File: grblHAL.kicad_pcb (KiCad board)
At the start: 2 copper layers, 48 parts, among them J1 Conn_01x03, J2 Conn_02x08_Odd_Even, J3 Conn_01x06, J4 Conn_01x06, J5 Conn_01x04, U1 YAAJ_BluePill_Part_Like_SWD_B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, U10 PC817, U11 PC817, U12 PC817, U13 PC817, U14 LM1117-3.3, U2 TMC2208_SILENTSTEPSTICK, U4 PC817, U5 PC817, U6 PC817, U7 PC817, U8 PC817, U9 PC817

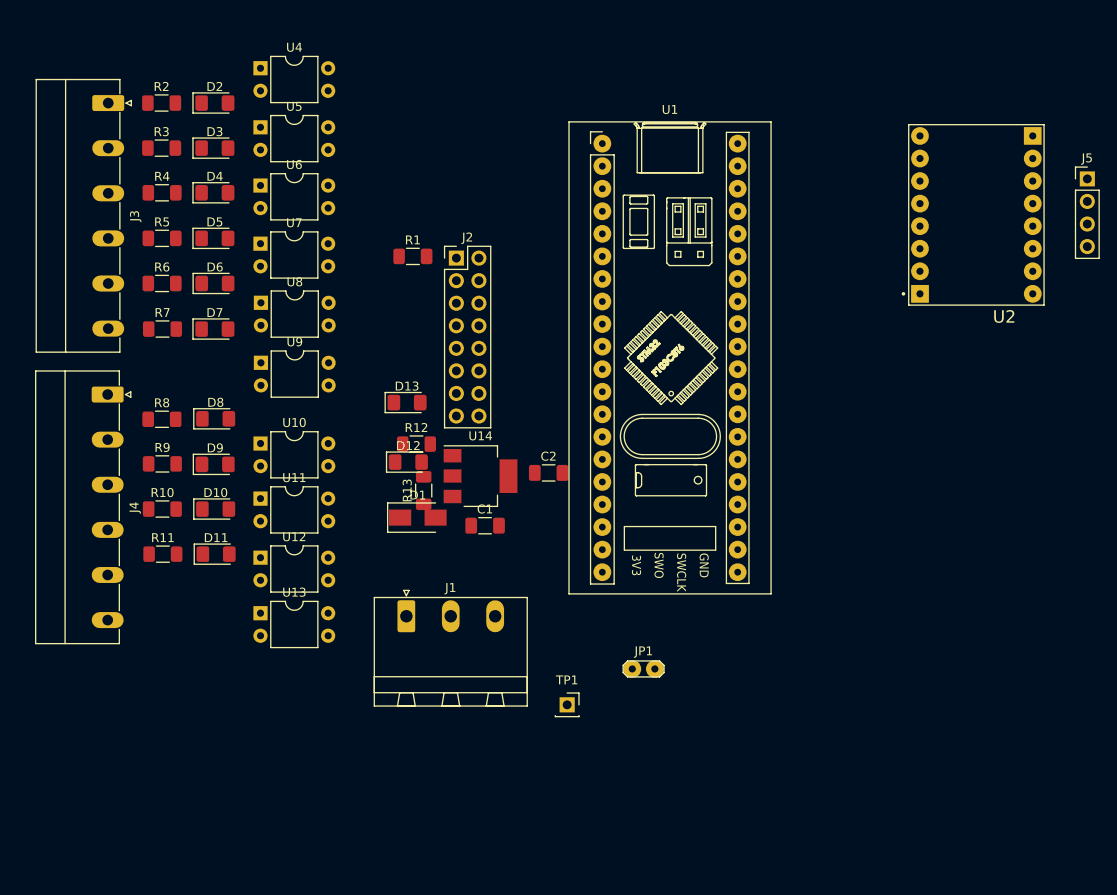
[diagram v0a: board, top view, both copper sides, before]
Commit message: Schematic Layout Nets Opto 4 TMC Stage 2
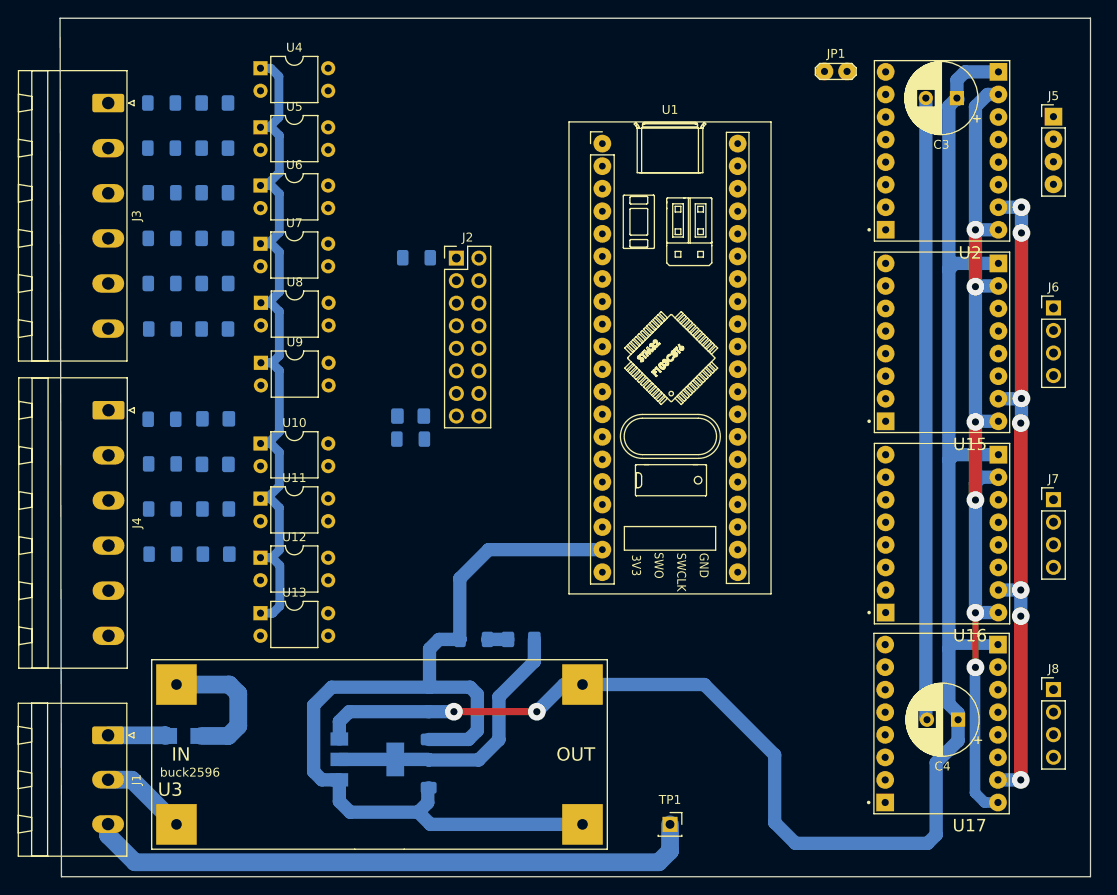
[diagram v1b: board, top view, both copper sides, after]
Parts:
- added C3: 100uF/35v, Capacitor_THT:CP_Radial_D8.0mm_P3.50mm, F.Cu at (156.1, 60.1)
- added C4: 100uF/35v, Capacitor_THT:CP_Radial_D8.0mm_P3.50mm, F.Cu at (156.2, 130.1)
- added J6: Conn_01x04, Connector_PinHeader_2.54mm:PinHeader_1x04_P2.54mm_Vertical, F.Cu at (166.9, 83.7)
- added J7: Conn_01x04, Connector_PinHeader_2.54mm:PinHeader_1x04_P2.54mm_Vertical, F.Cu at (166.9, 105.3)
- added J8: Conn_01x04, Connector_PinHeader_2.54mm:PinHeader_1x04_P2.54mm_Vertical, F.Cu at (166.9, 126.7)
- added U15: TMC2208, TMC2208_SILENTSTEPSTICK:MODULE_TMC2208_SILENTSTEPSTICK, F.Cu at (154.4, 87.6)
- added U16: TMC2208, TMC2208_SILENTSTEPSTICK:MODULE_TMC2208_SILENTSTEPSTICK, F.Cu at (154.4, 109.1)
- added U17: TMC2208, TMC2208_SILENTSTEPSTICK:MODULE_TMC2208_SILENTSTEPSTICK, F.Cu at (154.3, 130.5)
- added U3: buck2596, DC_DC_LM2596_small:DC_DC_LM2596_small, F.Cu at (91.0, 134.0)
- C1, C2, D1, D10, D11, D12, D13, D2, D3, D4, D5, D6, D7, D8, D9, R1, R10, R11, R12, R13, R2, R3, R4, R5, R6, R7, R8, R9, U14: moved to B.Cu
- J2: value Conn_02x08_Odd_Even -> Conn
- J3, J4: footprint Connector_Phoenix_MC_HighVoltage:PhoenixContact_MC_1,5_6-G-5.08_1x06_P5.08mm_Horizontal -> Connector_Phoenix_MSTB:PhoenixContact_MSTBA_2,5_6-G-5,08_1x06_P5.08mm_Horizontal
- U2: value TMC2208_SILENTSTEPSTICK -> TMC2208
- moved JP1 70.7 mm to (141.1, 57.1)
- moved C2 36.5 mm to (96.6, 136.2), turned to -90 degrees
- moved J1 36.2 mm to (60.5, 131.9), turned to -90 degrees
- moved D1 36.1 mm to (69.0, 131.9), turned to 180 degrees
- moved U14 34.4 mm to (89.7, 134.6)
- moved D12 23.7 mm to (107.0, 121.1)
- moved C1 23.4 mm to (96.6, 130.8), turned to -90 degrees
- moved TP1 17.8 mm to (123.7, 141.9)
- moved R13 17.7 mm to (101.7, 121.1), turned to 0 degrees
- moved U2 8.18 mm to (154.4, 66.0)
- moved J5 7.98 mm to (166.9, 62.2)
- moved J4 1.77 mm to (60.5, 95.2)
- moved D13 1.58 mm to (94.5, 95.9), turned to 180 degrees
- moved R12 0.87 mm to (94.5, 98.5)
- moved R1 0.43 mm to (95.2, 78.1)
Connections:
- C1 pad 2: 5V -> GND
- C2 pad 2: 5V -> GND
- JP1 pad 1: 5V -> GND
- JP1 pad 2: EN -> STEN
- R12 pad 1: 5V -> GND
- R13 pad 1: 5V -> GND
- U1 pad 19: 5V -> GND
- U1 pad 39: 5V -> GND
- U10 pad 3: 5V -> GND
- U11 pad 3: 5V -> GND
- U12 pad 3: 5V -> GND
- U13 pad 3: 5V -> GND
- U14 pad 1: 5V -> GND
- U2 pad JP1_8: EN -> STEN
- U2 pad JP2_2: 5V -> GND
- U2 pad JP2_8: 5V -> GND
- U4 pad 3: 5V -> GND
- U5 pad 3: 5V -> GND
- U6 pad 3: 5V -> GND
- U7 pad 3: 5V -> GND
- U8 pad 3: 5V -> GND
- U9 pad 3: 5V -> GND
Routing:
- net GND: track 0.00 -> 275.7 mm, vias 0 -> 6
- net VM: track 0.00 -> 192.7 mm, vias 0 -> 2
- net Net-(J4-Pad5): track 0.00 -> 88.4 mm
- net 3V3: track 0.00 -> 74.8 mm, vias 0 -> 7
- net Net-(J1-Pad3): track 0.00 -> 69.3 mm
- net 5V: track 0.00 -> 31.9 mm
- net Net-(D1-Pad1): track 0.00 -> 15.6 mm
- net Net-(J1-Pad2): track 0.00 -> 9.79 mm
- net Net-(D1-Pad2): track 0.00 -> 6.55 mm
- net Net-(D12-Pad1): track 0.00 -> 2.30 mm
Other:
- board outline added: 116 x 96.7 mm
